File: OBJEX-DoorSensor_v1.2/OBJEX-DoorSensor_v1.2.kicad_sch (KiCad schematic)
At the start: 32 parts, among them Q1 BC857B_RF, Q2 NTNUS3171PZT5G, U1 ESP32-C3-MINI-1-N4, U2 RT9080-33GJ5, U3 S-5701BC11B-L3T2U5, U4 SN74LVC1G86DBVR, U5 SN74LVC1G86DBVR, Y1 Crystal

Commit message: UPDATE
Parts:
- removed C1, C3: 10uF, Capacitor_SMD:C_0402_1005Metric, symbol Device:C
- removed C2: 0.1uF, Capacitor_SMD:C_0402_1005Metric, symbol Device:C
- removed C4, C5: 12pF, Capacitor_SMD:C_0402_1005Metric, symbol Device:C
- removed C6: 1uF, Capacitor_SMD:C_0603_1608Metric, symbol Device:C
- removed C7: 1uF/4.7uF, Capacitor_SMD:C_0603_1608Metric, symbol Device:C
- removed C8: 10uF, symbol Device:C
- removed C9: C, symbol Device:C
- removed JP1, JP2: SolderJumper_2_Bridged, Jumper:SolderJumper-2_P1.3mm_Bridged_RoundedPad1.0x1.5mm, symbol Jumper:SolderJumper_2_Bridged
- removed JP3: SolderJumper_2_Open, Jumper:SolderJumper-2_P1.3mm_Open_RoundedPad1.0x1.5mm, symbol Jumper:SolderJumper_2_Open
- removed Q1: BC857B_RF, SOT95P237X112-3N, symbol BC857B_RF:BC857B_RF
- removed Q2: NTNUS3171PZT5G, ONSC-SOT-1123-3-524AA_V, symbol NTNUS3171PZT5G:NTNUS3171PZT5G
- removed R1, R2, R3, R4: 10K, Resistor_SMD:R_0402_1005Metric, symbol Device:R
- removed R10, R8, R9: 10K, symbol Device:R
- removed R11: 1M, symbol Device:R
- removed R5: 100M, symbol Device:R
- removed R6, R7: R, symbol Device:R
- removed S1: MDSM-4R-12-18, MDSM4R1218, symbol MDSM-4R-12-18:MDSM-4R-12-18
- removed U1: ESP32-C3-MINI-1-N4, XCVR_ESP32-C3-MINI-1-N4, symbol ESP32-C3-MINI-1-N4:ESP32-C3-MINI-1-N4
- removed U2: RT9080-33GJ5, KicadLibrary:TSOT-23, symbol RT9080-33GJ5:RT9080-33GJ5
- removed U3: S-5701BC11B-L3T2U5, symbol Ablic_S-5701:S-5701BC11B-L3T2U5
- removed U4, U5: SN74LVC1G86DBVR, SOT353, symbol SN74LVC1G86DBVR:SN74LVC1G86DBVR
- removed Y1: Crystal, Crystal:Crystal_SMD_2012-2Pin_2.0x1.2mm, symbol Device:Crystal
- added TP1: BATT, symbol Connector:TestPoint
- added TP2: GND, symbol Connector:TestPoint
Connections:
- net +BATT: now also TP1.1
- net GND: now also TP2.1
- no-connect marks 1 -> 0
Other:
- added sheet BME680 (BME680.kicad_sch)
- added sheet LDO (RT9080.kicad_sch)
- added sheet Microcontroller + WiFi-BLE (esp32c3.kicad_sch)
- added sheet Power Latch - Transient signal detector (PowerLatch.kicad_sch)
- note added: "Terminal Battery x2 AAA"
- note removed: "D"
- note removed: "S"
- note removed: "VBAT = 3/3.3V ?"
- note removed: "uC AUTO TURN OFF"

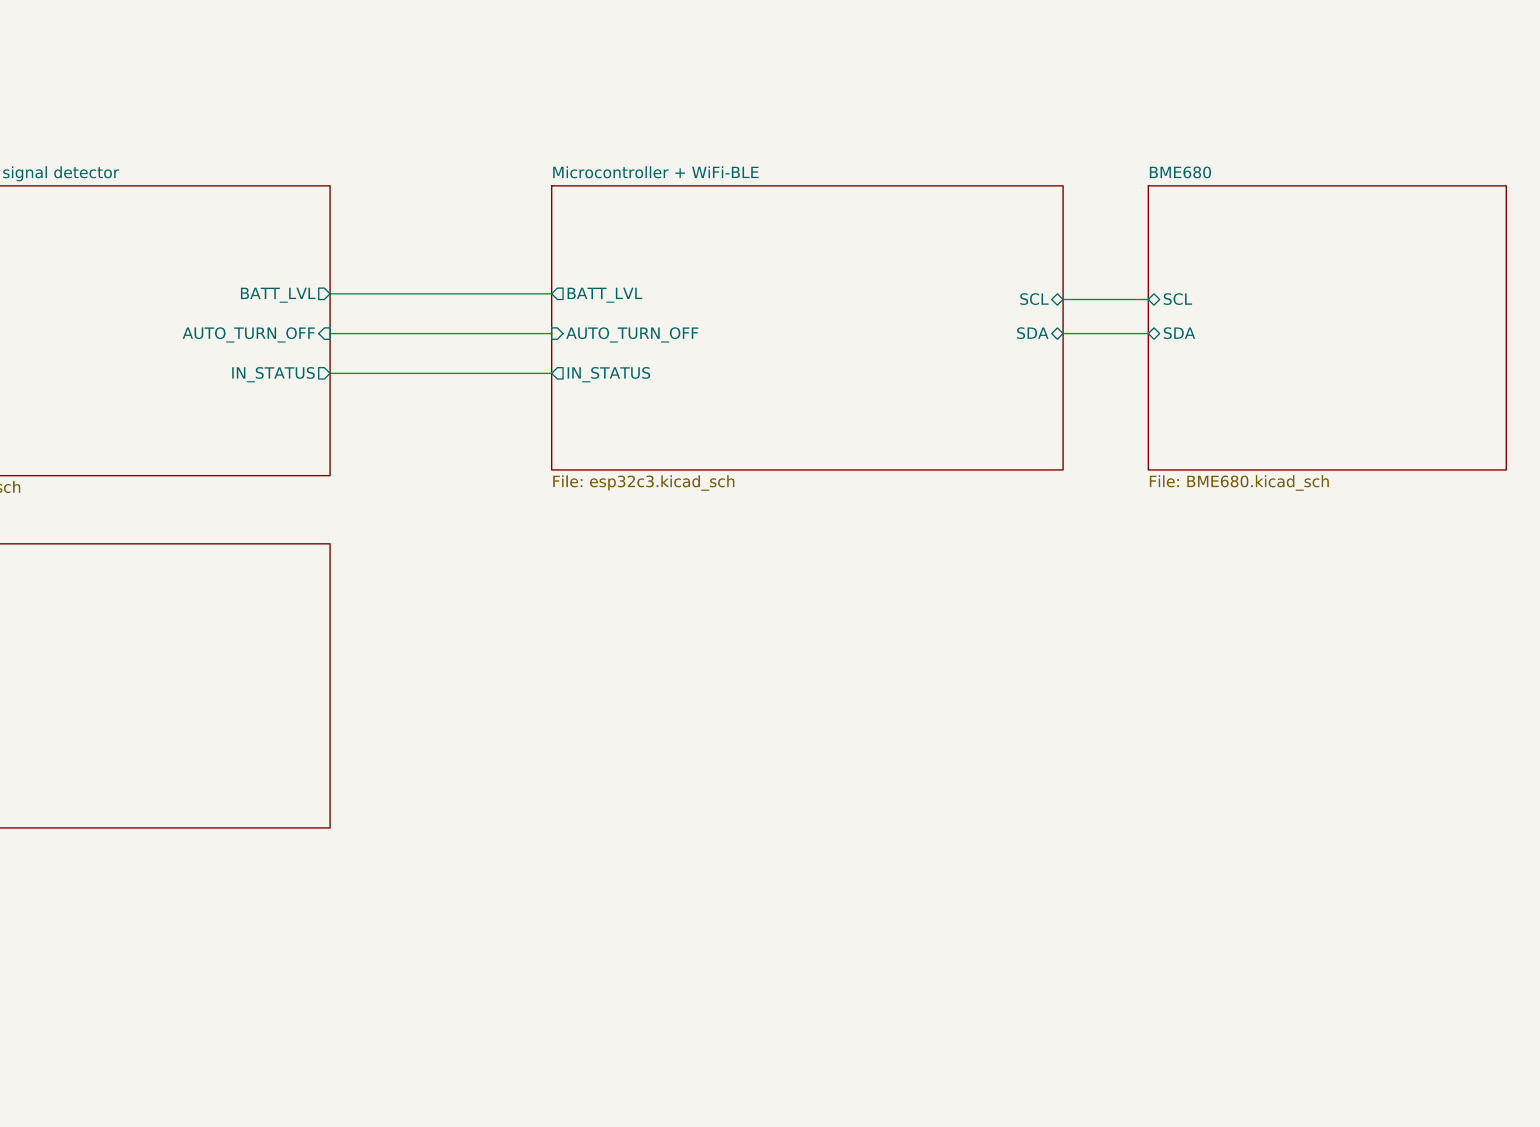
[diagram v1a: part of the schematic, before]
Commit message: SCH complate
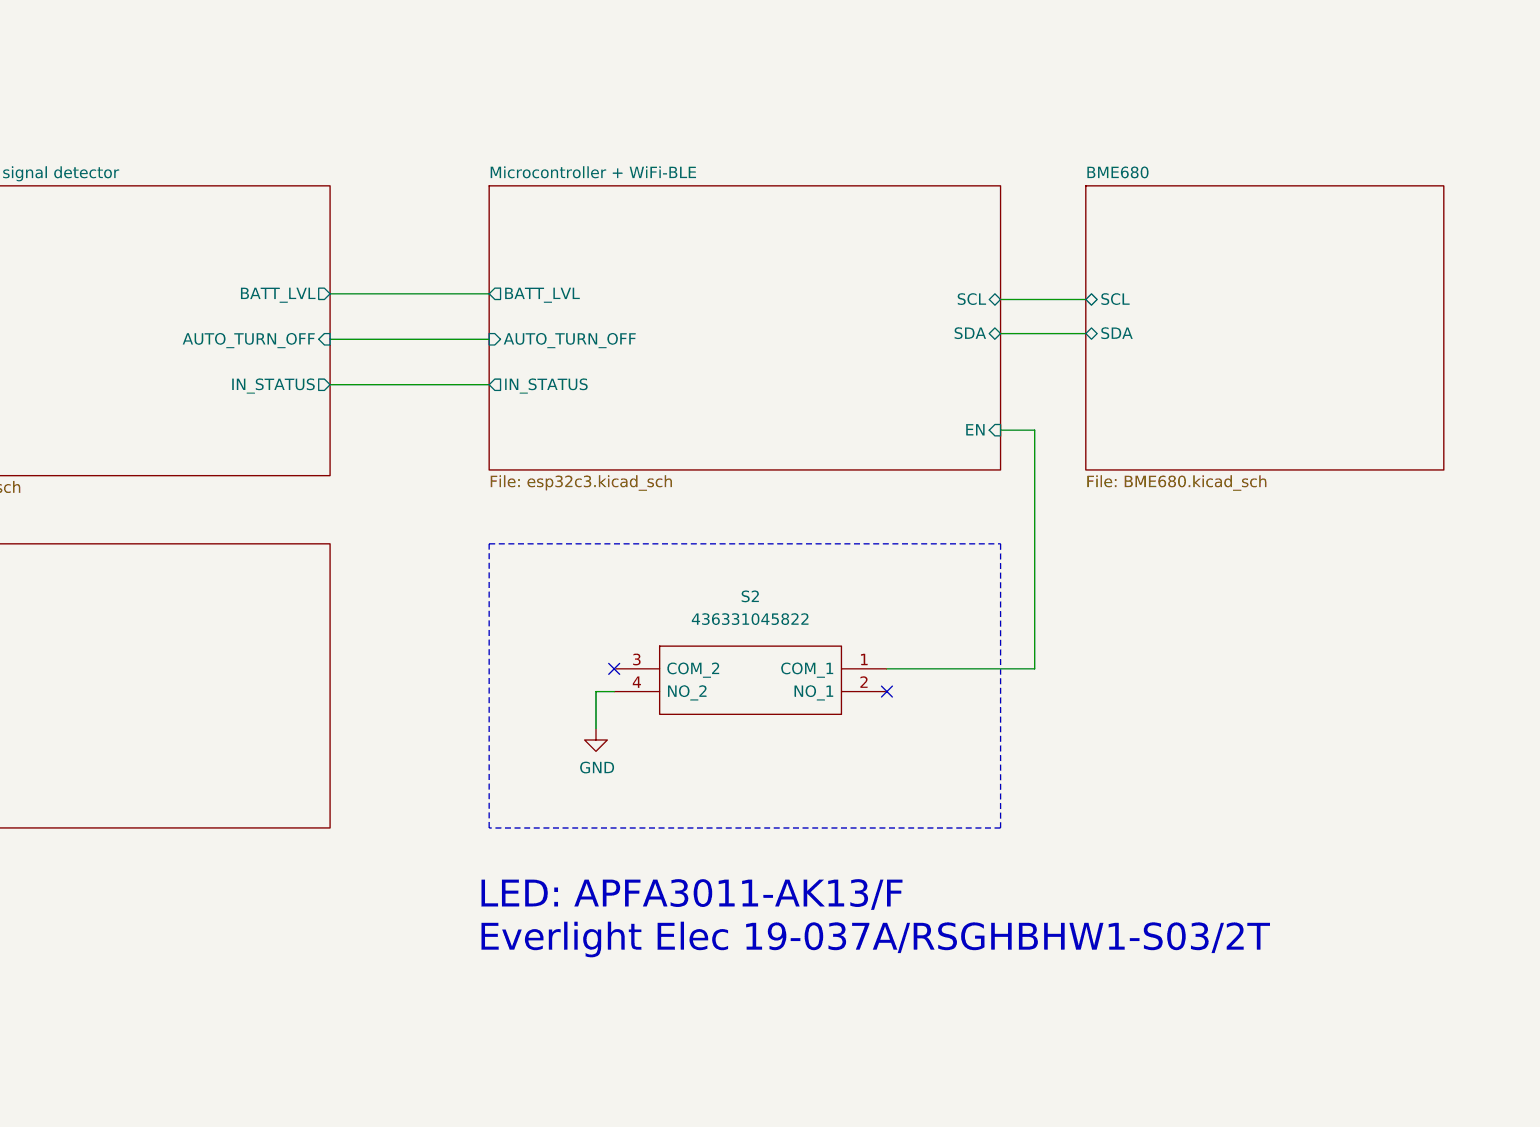
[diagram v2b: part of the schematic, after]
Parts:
- added S2: 436331045822, SamacSys_Parts:436331045822, symbol SamacSys_Parts:436331045822
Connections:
- net GND: now also S2.4 (NO_2)
- new net Microcontroller + WiFi-BLE/EN: S2.1 (COM_1)
- no-connect marks 0 -> 2
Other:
- sheet Microcontroller + WiFi-BLE ports: added EN; removed none
- note added: "LED: APFA3011-AK13/F Everlight Elec 19-037A/RSGHBHW1-S03/2T"
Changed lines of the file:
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@@
     (comment 2 "Designer: Salvatore Raccardi")
   )
-  (wire (pts (xy 124.46 79.375) (xy 149.225 79.375))
-    (stroke (width 0) (type default))
-  )
-  (wire (pts (xy 206.375 79.375) (xy 215.9 79.375))
-    (stroke (width 0) (type default))
-  )
-  (wire (pts (xy 206.375 75.565) (xy 215.9 75.565))
-    (stroke (width 0) (type default))
-  )
-  (wire (pts (xy 124.46 74.93) (xy 149.225 74.93))
+  (no_connect (at 186.69 119.38))
+  (no_connect (at 156.21 116.84))
+  (wire (pts (xy 124.46 80.01) (xy 142.24 80.01))
+    (stroke (width 0) (type default))
+  )
+  (wire (pts (xy 203.2 90.17) (xy 199.39 90.17))
+    (stroke (width 0) (type default))
+  )
+  (wire (pts (xy 199.39 79.375) (xy 208.915 79.375))
+    (stroke (width 0) (type default))
+  )
+  (wire (pts (xy 186.69 116.84) (xy 203.2 116.84))
+    (stroke (width 0) (type default))
+  )
+  (wire (pts (xy 199.39 75.565) (xy 208.915 75.565))
     (stroke (width 0) (type default))
   )
@@
     (stroke (width 0) (type default))
   )
+  (wire (pts (xy 203.2 116.84) (xy 203.2 90.17))
+    (stroke (width 0) (type default))
+  )
+  (wire (pts (xy 156.21 119.38) (xy 154.178 119.38))
+    (stroke (width 0) (type default))
+  )
   (wire (pts (xy 57.15 85.09) (xy 57.15 88.265))
     (stroke (width 0) (type default))
   )
+  (wire (pts (xy 124.46 85.09) (xy 142.24 85.09))
+    (stroke (width 0) (type default))
+  )
+  (wire (pts (xy 154.178 119.38) (xy 154.178 123.5202))
+    (stroke (width 0) (type default))
+  )
   (wire (pts (xy 52.07 85.09) (xy 57.15 85.09))
-    (stroke (width 0) (type default))
-  )
-  (wire (pts (xy 124.46 83.82) (xy 149.225 83.82))
     (stroke (width 0) (type default))
   )
@@
   (polyline (pts (xy 63.5 62.865) (xy 38.1 62.865))
     (stroke (width 0) (type dash_dot))
+  )
+  (wire (pts (xy 124.46 74.93) (xy 142.24 74.93))
+    (stroke (width 0) (type default))
+  )
+  (rectangle (start 142.24 102.87) (end 199.39 134.62)
+    (stroke (width 0) (type dash))
+    (fill (type none))
   )
   (image (at 263.2456 172.6692) (scale 0.510674)
@@
     (effects (font (size 1.2 1.2)) (justify left bottom))
   )
+  (text "LED: APFA3011-AK13/F\nEverlight Elec 19-037A/RSGHBHW1-S03/2T\n\n"
+    (at 140.97 153.67 0)
+    (effects (font (size 3 3)) (justify left bottom))
+  )
   (text "Terminal\nBattery x2 AAA" (at 38.1 61.595 0)
     (effects (font (size 2 2) (thickness 0.254) bold) (justify left bottom))
@@
     )
   )
+  (symbol (lib_id "power:GND") (at 154.178 123.5202 0) (unit 1)
+    (in_bom yes) (on_board yes) (dnp no)
+    (property "Reference" "#PWR010" (at 154.178 129.8702 0)
+      (effects (font (size 1.27 1.27)) hide)
+    )
+    (property "Value" "GND" (at 154.305 127.9144 0)
+      (effects (font (size 1.27 1.27)))
+    )
+    (property "Footprint" "" (at 154.178 123.5202 0)
+      (effects (font (size 1.27 1.27)) hide)
+    )
+    (property "Datasheet" "" (at 154.178 123.5202 0)
+      (effects (font (size 1.27 1.27)) hide)
+    )
+    (pin "1")
+    (instances
+      (project "OBJEX-DoorSensor_v1.2"
+        (path "/dfd7f005-123d-49c6-a596-950b92e8aba7"
+          (reference "#PWR010") (unit 1)
+        )
+      )
+    )
+  )
   (symbol (lib_id "Connector:TestPoint") (at 52.07 73.025 90) (unit 1)
     (in_bom yes) (on_board yes) (dnp no)
@@
         (path "/dfd7f005-123d-49c6-a596-950b92e8aba7"
           (reference "TP1") (unit 1)
+        )
+      )
+    )
+  )
+  (symbol (lib_id "SamacSys_Parts:436331045822") (at 156.21 116.84 0) (unit 1)
+    (in_bom yes) (on_board yes) (dnp no) (fields_autoplaced)
+    (property "Reference" "S2" (at 171.45 108.7882 0)
+      (effects (font (size 1.27 1.27)))
+    )
+    (property "Value" "436331045822" (at 171.45 111.3282 0)
+      (effects (font (size 1.27 1.27)))
+    )
+    (property "Footprint" "SamacSys_Parts:436331045822" (at 182.88 114.3 0)
+      (effects (font (size 1.27 1.27)) (justify left) hide)
+    )
+    (property "Datasheet" "http://katalog.we-online.de/em/datasheet/4363x10458xx.pdf" (at 182.88 116.84 0)
+      (effects (font (size 1.27 1.27)) (justify left) hide)
+    )
+    (property "Description" "Black Tactile Switch, NO 50 mA@ 12 V dc 2.6mm Surface Mount" (at 182.88 119.38 0)
+      (effects (font (size 1.27 1.27)) (justify left) hide)
+    )
+    (property "Height" "1.65" (at 182.88 121.92 0)
+      (effects (font (size 1.27 1.27)) (justify left) hide)
+    )
+    (property "Mouser Part Number" "710-436331045822" (at 182.88 124.46 0)
+      (effects (font (size 1.27 1.27)) (justify left) hide)
+    )
+    (property "Mouser Price/Stock" "https://www.mouser.co.uk/ProductDetail/Wurth-Elektronik/436331045822?qs=wr8lucFkNMXz9UbduBxtIQ%3D%3D" (at 182.88 127 0)
+      (effects (font (size 1.27 1.27)) (justify left) hide)
+    )
+    (property "Manufacturer_Name" "Wurth Elektronik" (at 182.88 129.54 0)
+      (effects (font (size 1.27 1.27)) (justify left) hide)
+    )
+    (property "Manufacturer_Part_Number" "436331045822" (at 182.88 132.08 0)
+      (effects (font (size 1.27 1.27)) (justify left) hide)
+    )
+    (pin "1")
+    (pin "2")
+    (pin "3")
+    (pin "4")
+    (instances
+      (project "OBJEX-DoorSensor_v1.2"
+        (path "/dfd7f005-123d-49c6-a596-950b92e8aba7"
+          (reference "S2") (unit 1)
         )
       )
@@
     )
   )
-  (sheet (at 149.225 62.865) (size 57.15 31.75) (fields_autoplaced)
+  (sheet (at 142.24 62.865) (size 57.15 31.75) (fields_autoplaced)
     (stroke (width 0.1524) (type solid))
     (fill (color 0 0 0 0.0000))
-    (property "Sheetname" "Microcontroller + WiFi-BLE" (at 149.225 62.1534 0)
+    (property "Sheetname" "Microcontroller + WiFi-BLE" (at 142.24 62.1534 0)
       (effects (font (size 1.27 1.27)) (justify left bottom))
     )
-    (property "Sheetfile" "esp32c3.kicad_sch" (at 149.225 95.1996 0)
+    (property "Sheetfile" "esp32c3.kicad_sch" (at 142.24 95.1996 0)
       (effects (font (size 1.27 1.27)) (justify left top))
     )
-    (property "Field2" "" (at 149.225 62.865 0)
-      (effects (font (size 1.27 1.27)) hide)
-    )
-    (pin "BATT_LVL" output (at 149.225 74.93 180)
+    (property "Field2" "" (at 142.24 62.865 0)
+      (effects (font (size 1.27 1.27)) hide)
+    )
+    (pin "BATT_LVL" output (at 142.24 74.93 180)
       (effects (font (size 1.27 1.27)) (justify left))
     )
-    (pin "AUTO_TURN_OFF" input (at 149.225 79.375 180)
+    (pin "AUTO_TURN_OFF" input (at 142.24 80.01 180)
       (effects (font (size 1.27 1.27)) (justify left))
     )
-    (pin "IN_STATUS" output (at 149.225 83.82 180)
+    (pin "IN_STATUS" output (at 142.24 85.09 180)
       (effects (font (size 1.27 1.27)) (justify left))
     )
-    (pin "SDA" bidirectional (at 206.375 79.375 0)
+    (pin "SDA" bidirectional (at 199.39 79.375 0)
       (effects (font (size 1.27 1.27)) (justify right))
     )
-    (pin "SCL" bidirectional (at 206.375 75.565 0)
+    (pin "SCL" bidirectional (at 199.39 75.565 0)
+      (effects (font (size 1.27 1.27)) (justify right))
+    )
+    (pin "EN" input (at 199.39 90.17 0)
       (effects (font (size 1.27 1.27)) (justify right))
     )
@@
       (effects (font (size 1.27 1.27)) (justify right))
     )
-    (pin "AUTO_TURN_OFF" input (at 124.46 79.375 0)
+    (pin "AUTO_TURN_OFF" input (at 124.46 80.01 0)
       (effects (font (size 1.27 1.27)) (justify right))
     )
-    (pin "IN_STATUS" output (at 124.46 83.82 0)
+    (pin "IN_STATUS" output (at 124.46 85.09 0)
       (effects (font (size 1.27 1.27)) (justify right))
     )
@@
     )
   )
-  (sheet (at 215.9 62.865) (size 40.005 31.75) (fields_autoplaced)
+  (sheet (at 208.915 62.865) (size 40.005 31.75) (fields_autoplaced)
     (stroke (width 0.1524) (type solid))
     (fill (color 0 0 0 0.0000))
-    (property "Sheetname" "BME680" (at 215.9 62.1534 0)
+    (property "Sheetname" "BME680" (at 208.915 62.1534 0)
       (effects (font (size 1.27 1.27)) (justify left bottom))
     )
-    (property "Sheetfile" "BME680.kicad_sch" (at 215.9 95.1996 0)
+    (property "Sheetfile" "BME680.kicad_sch" (at 208.915 95.1996 0)
       (effects (font (size 1.27 1.27)) (justify left top))
     )
-    (pin "SCL" bidirectional (at 215.9 75.565 180)
+    (pin "SCL" bidirectional (at 208.915 75.565 180)
       (effects (font (size 1.27 1.27)) (justify left))
     )
-    (pin "SDA" bidirectional (at 215.9 79.375 180)
+    (pin "SDA" bidirectional (at 208.915 79.375 180)
       (effects (font (size 1.27 1.27)) (justify left))
     )
